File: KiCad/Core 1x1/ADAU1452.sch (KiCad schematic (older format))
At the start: 71 parts, among them Q1 2STF2550, U7 ADAU1452, U8 M95M01, Y1 12.288MHz

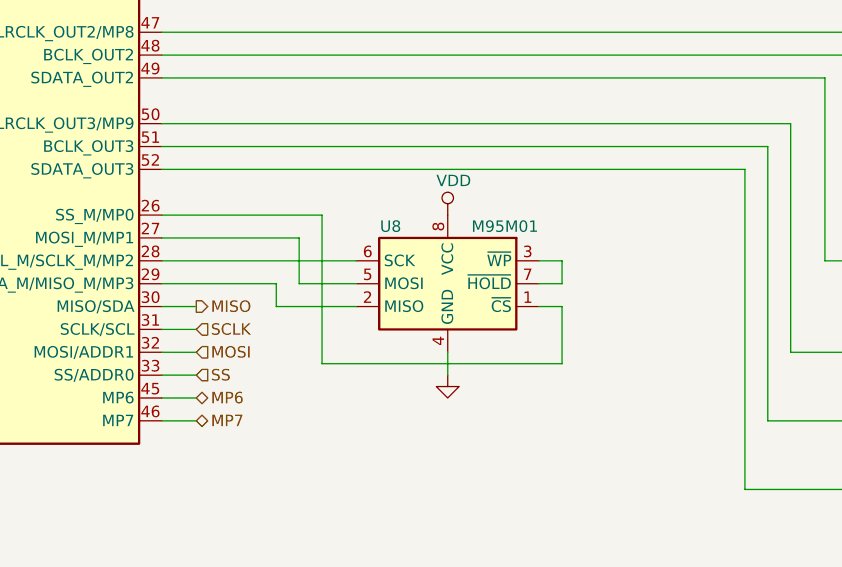
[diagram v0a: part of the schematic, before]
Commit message: Progress Commit
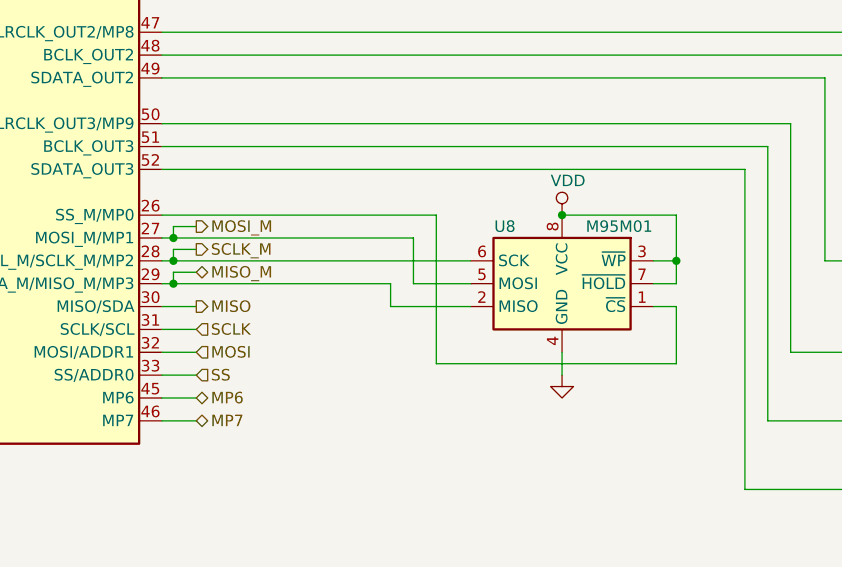
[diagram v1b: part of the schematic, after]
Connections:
- net VDD: now also U8.3 (~WP), U8.7 (~HOLD)
- net MOSI_M: now reaches U7.27 (MOSI_M/MP1), U8.5 (MOSI)
- net SCLK_M: now reaches U7.28 (SCL_M/SCLK_M/MP2), U8.6 (SCK)
- net MISO_M: now reaches U7.29 (SDA_M/MISO_M/MP3), U8.2 (MISO)
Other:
- moved on the sheet: U8
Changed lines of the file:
@@
 Wire Wire Line
 	13200 3450 13350 3450
-$Comp
-L power:VDD #PWR0145
-U 1 1 5E15EEA5
-P 10500 6150
-F 0 "#PWR0145" H 10500 6000 50  0001 C CNN
-F 1 "VDD" H 10450 6300 50  0000 L CNN
-F 2 "" H 10500 6150 50  0001 C CNN
-F 3 "" H 10500 6150 50  0001 C CNN
-	1    10500 6150
-	1    0    0    -1
-$EndComp
 Text HLabel 6350 6150 0    50   Input ~ 0
 SELFBOOT
@@
 MP7
 Wire Wire Line
-	10500 6850 10500 6750
+	11000 6850 11000 6750
 $Comp
 L power:GND #PWR0149
 U 1 1 5E8FCA37
-P 10500 6850
-F 0 "#PWR0149" H 10500 6600 50  0001 C CNN
-F 1 "GND" H 10505 6677 50  0001 C CNN
-F 2 "" H 10500 6850 50  0001 C CNN
-F 3 "" H 10500 6850 50  0001 C CNN
-	1    10500 6850
+P 11000 6850
+F 0 "#PWR0149" H 11000 6600 50  0001 C CNN
+F 1 "GND" H 11005 6677 50  0001 C CNN
+F 2 "" H 11000 6850 50  0001 C CNN
+F 3 "" H 11000 6850 50  0001 C CNN
+	1    11000 6850
 	1    0    0    -1
 $EndComp
@@
 L Memory_EEPROM:25LCxxx U8
 U 1 1 5EB9D283
-P 10500 6450
-F 0 "U8" H 10750 6700 50  0000 C CNN
-F 1 "M95M01" H 10250 6700 50  0000 C CNN
-F 2 "Package_SO:SO-8_3.9x4.9mm_P1.27mm" H 10500 6450 50  0001 C CNN
-F 3 "http://ww1.microchip.com/downloads/en/DeviceDoc/21832H.pdf" H 10500 6450 50  0001 C CNN
-	1    10500 6450
+P 11000 6450
+F 0 "U8" H 11250 6700 50  0000 C CNN
+F 1 "M95M01" H 10750 6700 50  0000 C CNN
+F 2 "Package_SO:SO-8_3.9x4.9mm_P1.27mm" H 11000 6450 50  0001 C CNN
+F 3 "http://ww1.microchip.com/downloads/en/DeviceDoc/21832H.pdf" H 11000 6450 50  0001 C CNN
+	1    11000 6450
 	-1   0    0    -1
 $EndComp
@@
 	11800 5950 11800 7350
 Wire Wire Line
-	10900 6350 11000 6350
-Wire Wire Line
-	10900 6450 11000 6450
-Wire Wire Line
-	11000 6350 11000 6450
-Wire Wire Line
-	9250 6150 9950 6150
-Wire Wire Line
-	9950 6800 11000 6800
-Wire Wire Line
-	11000 6800 11000 6550
-Wire Wire Line
-	11000 6550 10900 6550
-Wire Wire Line
-	9950 6150 9950 6800
-Wire Wire Line
-	9250 6250 9850 6250
-Wire Wire Line
-	9850 6250 9850 6450
-Wire Wire Line
-	9850 6450 10100 6450
-Wire Wire Line
-	9250 6350 10100 6350
-Wire Wire Line
-	9250 6450 9750 6450
-Wire Wire Line
-	9750 6450 9750 6550
-Wire Wire Line
-	9750 6550 10100 6550
+	11400 6350 11500 6350
+Wire Wire Line
+	11400 6450 11500 6450
+Wire Wire Line
+	11500 6350 11500 6450
+Wire Wire Line
+	10450 6800 11500 6800
+Wire Wire Line
+	11500 6800 11500 6550
+Wire Wire Line
+	11500 6550 11400 6550
+Wire Wire Line
+	10450 6150 10450 6800
+Wire Wire Line
+	10350 6250 10350 6450
+Wire Wire Line
+	10350 6450 10600 6450
+Wire Wire Line
+	10250 6450 10250 6550
+Wire Wire Line
+	10250 6550 10600 6550
 Text HLabel 9400 6550 2    50   Output ~ 0
 MISO
@@
 	5450 2150 6650 2150
 Connection ~ 5450 2700
+Wire Wire Line
+	9250 6250 9300 6250
+Wire Wire Line
+	9250 6350 9300 6350
+Wire Wire Line
+	9250 6450 9300 6450
+Text HLabel 9400 6400 2    50   BiDi ~ 0
+MISO_M
+Text HLabel 9400 6300 2    50   Output ~ 0
+SCLK_M
+Text HLabel 9400 6200 2    50   Output ~ 0
+MOSI_M
+Wire Wire Line
+	9300 6450 9300 6400
+Wire Wire Line
+	9300 6400 9400 6400
+Connection ~ 9300 6450
+Wire Wire Line
+	9300 6450 10250 6450
+Wire Wire Line
+	9300 6350 9300 6300
+Wire Wire Line
+	9300 6300 9400 6300
+Connection ~ 9300 6350
+Wire Wire Line
+	9300 6350 10600 6350
+Wire Wire Line
+	9300 6250 9300 6200
+Wire Wire Line
+	9300 6200 9400 6200
+Connection ~ 9300 6250
+Wire Wire Line
+	9300 6250 10350 6250
+Wire Wire Line
+	9250 6150 10450 6150
+$Comp
+L power:VDD #PWR0145
+U 1 1 5E15EEA5
+P 11000 6150
+F 0 "#PWR0145" H 11000 6000 50  0001 C CNN
+F 1 "VDD" H 10950 6300 50  0000 L CNN
+F 2 "" H 11000 6150 50  0001 C CNN
+F 3 "" H 11000 6150 50  0001 C CNN
+	1    11000 6150
+	1    0    0    -1
+$EndComp
+Wire Wire Line
+	11500 6350 11500 6150
+Wire Wire Line
+	11500 6150 11000 6150
+Connection ~ 11500 6350
+Connection ~ 11000 6150
 $EndSCHEMATC
